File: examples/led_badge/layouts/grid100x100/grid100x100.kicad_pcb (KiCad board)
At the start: 4 copper layers, 200 parts

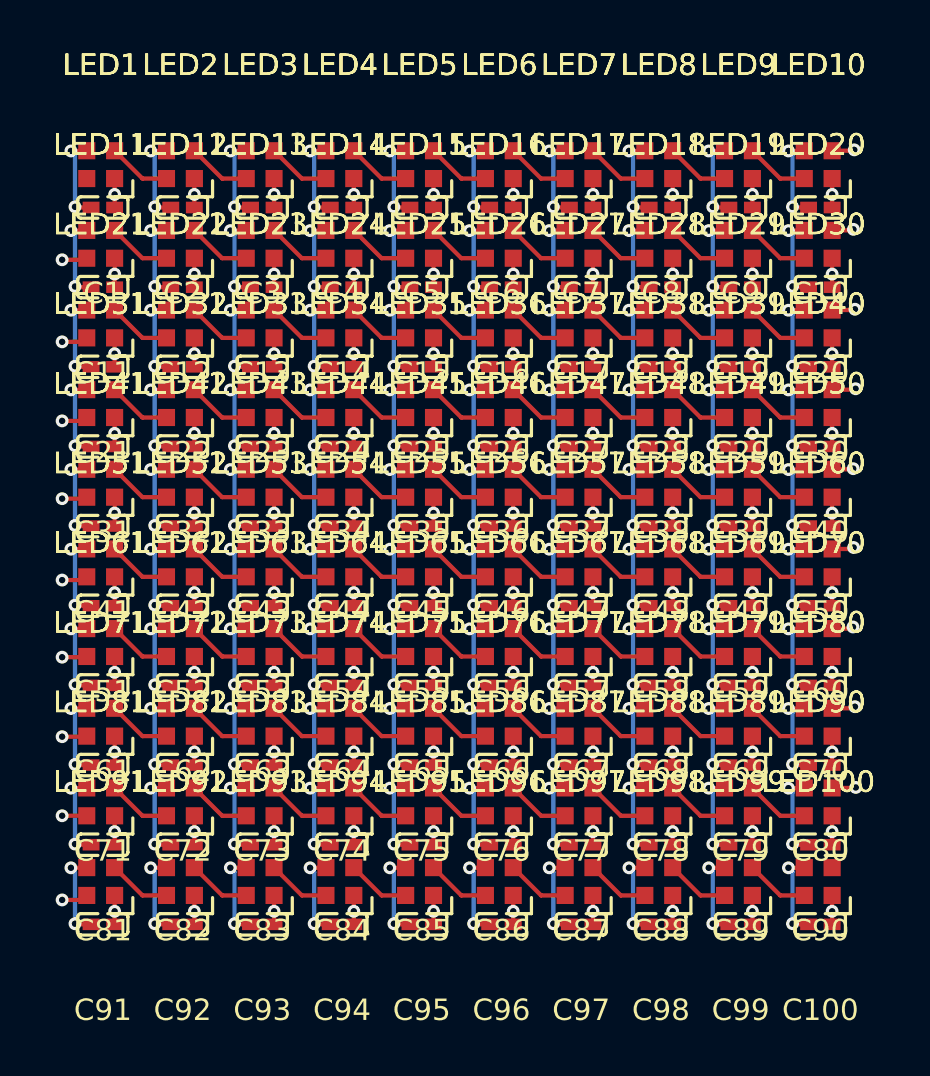
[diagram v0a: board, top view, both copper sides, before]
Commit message: just need usb to work
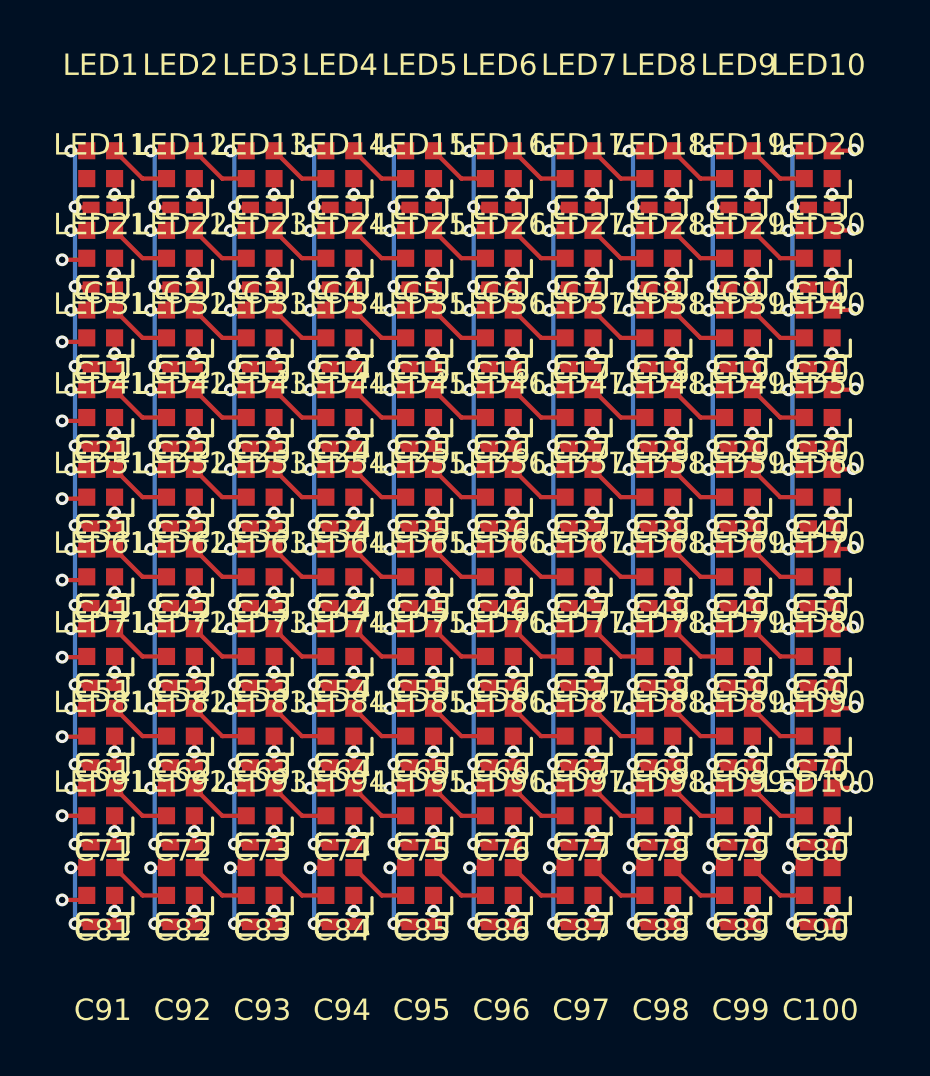
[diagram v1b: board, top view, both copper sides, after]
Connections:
- net -line-0 renamed rows[0]-data_in-line
- net -line-1 renamed data_out-line
- net -line-10 renamed rows[9]-data_in-line
- net -line-2 renamed rows[1]-data_in-line
- net -line-3 renamed rows[2]-data_in-line
- net -line-4 renamed rows[3]-data_in-line
- net -line-5 renamed rows[4]-data_in-line
- net -line-6 renamed rows[5]-data_in-line
- net -line-7 renamed rows[6]-data_in-line
- net -line-8 renamed rows[7]-data_in-line
- net -line-9 renamed rows[8]-data_in-line
- net gnd renamed GND
- net hv renamed VCC
- net rows[0]-DOUT-0 renamed leds[1]-data_in-DIN-0
- net rows[0]-DOUT-1 renamed leds[2]-data_in-DIN-0
- net rows[0]-DOUT-2 renamed leds[3]-data_in-DIN-0
- net rows[0]-DOUT-3 renamed leds[4]-data_in-DIN-0
- net rows[0]-DOUT-4 renamed leds[5]-data_in-DIN-0
- net rows[0]-DOUT-5 renamed leds[6]-data_in-DIN-0
- net rows[0]-DOUT-6 renamed leds[7]-data_in-DIN-0
- net rows[0]-DOUT-7 renamed leds[8]-data_in-DIN-0
- net rows[0]-DOUT-8 renamed leds[9]-data_in-DIN-0
- net rows[1]-DOUT-0 renamed leds[1]-data_in-DIN-1
- net rows[1]-DOUT-1 renamed leds[2]-data_in-DIN-1
- net rows[1]-DOUT-2 renamed leds[3]-data_in-DIN-1
- net rows[1]-DOUT-3 renamed leds[4]-data_in-DIN-1
- net rows[1]-DOUT-4 renamed leds[5]-data_in-DIN-1
- net rows[1]-DOUT-5 renamed leds[6]-data_in-DIN-1
- net rows[1]-DOUT-6 renamed leds[7]-data_in-DIN-1
- net rows[1]-DOUT-7 renamed leds[8]-data_in-DIN-1
- net rows[1]-DOUT-8 renamed leds[9]-data_in-DIN-1
- net rows[2]-DOUT-0 renamed leds[1]-data_in-DIN-2
- net rows[2]-DOUT-1 renamed leds[2]-data_in-DIN-2
- net rows[2]-DOUT-2 renamed leds[3]-data_in-DIN-2
- net rows[2]-DOUT-3 renamed leds[4]-data_in-DIN-2
- net rows[2]-DOUT-4 renamed leds[5]-data_in-DIN-2
- net rows[2]-DOUT-5 renamed leds[6]-data_in-DIN-2
- net rows[2]-DOUT-6 renamed leds[7]-data_in-DIN-2
- net rows[2]-DOUT-7 renamed leds[8]-data_in-DIN-2
- net rows[2]-DOUT-8 renamed leds[9]-data_in-DIN-2
- net rows[3]-DOUT-0 renamed leds[1]-data_in-DIN-3
- net rows[3]-DOUT-1 renamed leds[2]-data_in-DIN-3
- net rows[3]-DOUT-2 renamed leds[3]-data_in-DIN-3
- net rows[3]-DOUT-3 renamed leds[4]-data_in-DIN-3
- net rows[3]-DOUT-4 renamed leds[5]-data_in-DIN-3
- net rows[3]-DOUT-5 renamed leds[6]-data_in-DIN-3
- net rows[3]-DOUT-6 renamed leds[7]-data_in-DIN-3
- net rows[3]-DOUT-7 renamed leds[8]-data_in-DIN-3
- net rows[3]-DOUT-8 renamed leds[9]-data_in-DIN-3
- net rows[4]-DOUT-0 renamed leds[1]-data_in-DIN-4
- net rows[4]-DOUT-1 renamed leds[2]-data_in-DIN-4
- net rows[4]-DOUT-2 renamed leds[3]-data_in-DIN-4
- net rows[4]-DOUT-3 renamed leds[4]-data_in-DIN-4
- net rows[4]-DOUT-4 renamed leds[5]-data_in-DIN-4
- net rows[4]-DOUT-5 renamed leds[6]-data_in-DIN-4
- net rows[4]-DOUT-6 renamed leds[7]-data_in-DIN-4
- net rows[4]-DOUT-7 renamed leds[8]-data_in-DIN-4
- net rows[4]-DOUT-8 renamed leds[9]-data_in-DIN-4
- net rows[5]-DOUT-0 renamed leds[1]-data_in-DIN-5
- net rows[5]-DOUT-1 renamed leds[2]-data_in-DIN-5
- net rows[5]-DOUT-2 renamed leds[3]-data_in-DIN-5
- net rows[5]-DOUT-3 renamed leds[4]-data_in-DIN-5
- net rows[5]-DOUT-4 renamed leds[5]-data_in-DIN-5
- net rows[5]-DOUT-5 renamed leds[6]-data_in-DIN-5
- net rows[5]-DOUT-6 renamed leds[7]-data_in-DIN-5
- net rows[5]-DOUT-7 renamed leds[8]-data_in-DIN-5
- net rows[5]-DOUT-8 renamed leds[9]-data_in-DIN-5
- net rows[6]-DOUT-0 renamed leds[1]-data_in-DIN-6
- net rows[6]-DOUT-1 renamed leds[2]-data_in-DIN-6
- net rows[6]-DOUT-2 renamed leds[3]-data_in-DIN-6
- net rows[6]-DOUT-3 renamed leds[4]-data_in-DIN-6
- net rows[6]-DOUT-4 renamed leds[5]-data_in-DIN-6
- net rows[6]-DOUT-5 renamed leds[6]-data_in-DIN-6
- net rows[6]-DOUT-6 renamed leds[7]-data_in-DIN-6
- net rows[6]-DOUT-7 renamed leds[8]-data_in-DIN-6
- net rows[6]-DOUT-8 renamed leds[9]-data_in-DIN-6
- net rows[7]-DOUT-0 renamed leds[1]-data_in-DIN-7
- net rows[7]-DOUT-1 renamed leds[2]-data_in-DIN-7
- net rows[7]-DOUT-2 renamed leds[3]-data_in-DIN-7
- net rows[7]-DOUT-3 renamed leds[4]-data_in-DIN-7
- net rows[7]-DOUT-4 renamed leds[5]-data_in-DIN-7
- net rows[7]-DOUT-5 renamed leds[6]-data_in-DIN-7
- net rows[7]-DOUT-6 renamed leds[7]-data_in-DIN-7
- net rows[7]-DOUT-7 renamed leds[8]-data_in-DIN-7
- net rows[7]-DOUT-8 renamed leds[9]-data_in-DIN-7
- net rows[8]-DOUT-0 renamed leds[1]-data_in-DIN-8
- net rows[8]-DOUT-1 renamed leds[2]-data_in-DIN-8
- net rows[8]-DOUT-2 renamed leds[3]-data_in-DIN-8
- net rows[8]-DOUT-3 renamed leds[4]-data_in-DIN-8
- net rows[8]-DOUT-4 renamed leds[5]-data_in-DIN-8
- net rows[8]-DOUT-5 renamed leds[6]-data_in-DIN-8
- net rows[8]-DOUT-6 renamed leds[7]-data_in-DIN-8
- net rows[8]-DOUT-7 renamed leds[8]-data_in-DIN-8
- net rows[8]-DOUT-8 renamed leds[9]-data_in-DIN-8
- net rows[9]-DOUT-0 renamed leds[1]-data_in-DIN-9
- net rows[9]-DOUT-1 renamed leds[2]-data_in-DIN-9
- net rows[9]-DOUT-2 renamed leds[3]-data_in-DIN-9
- net rows[9]-DOUT-3 renamed leds[4]-data_in-DIN-9
- net rows[9]-DOUT-4 renamed leds[5]-data_in-DIN-9
- net rows[9]-DOUT-5 renamed leds[6]-data_in-DIN-9
- net rows[9]-DOUT-6 renamed leds[7]-data_in-DIN-9
- net rows[9]-DOUT-7 renamed leds[8]-data_in-DIN-9
- net rows[9]-DOUT-8 renamed leds[9]-data_in-DIN-9
